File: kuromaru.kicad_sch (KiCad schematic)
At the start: 63 parts, among them J1 USB_C_Receptacle_USB2.0, J102 Serial, J5 Conn_01x02, SW1 SW_Push, SW2 SW_Push, U1 RP2040, U2 GD25Q80CEIGR, U3 XC6210B332MR-G, U4 25LCxxx, Y1 Crystal_GND24

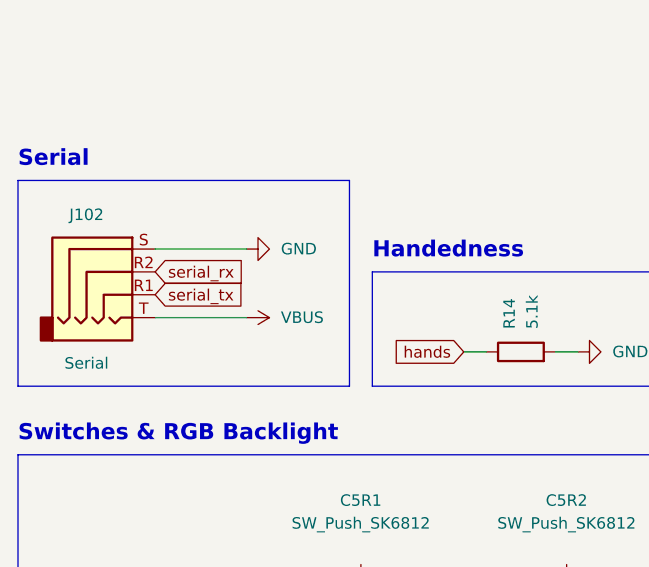
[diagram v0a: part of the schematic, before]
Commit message: Fix serial connector
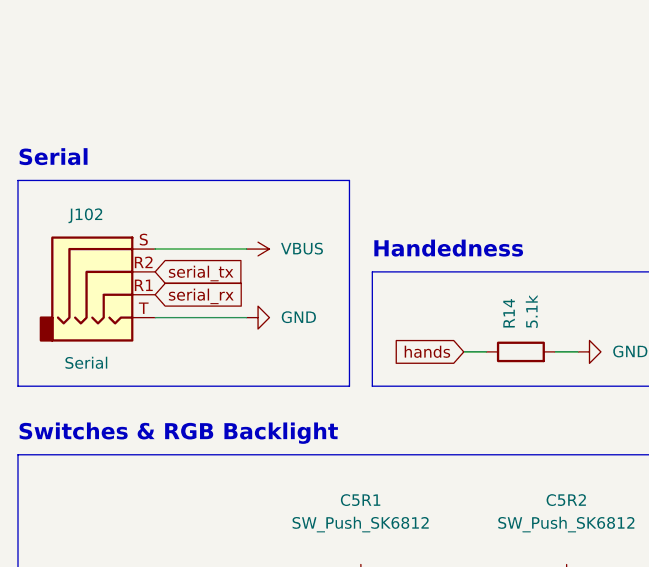
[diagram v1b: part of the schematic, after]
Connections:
- net GND: now also J102.T; no longer J102.S
- net VBUS: now also J102.S; no longer J102.T
- net serial_rx: now also J102.R1; no longer J102.R2
- net serial_tx: now also J102.R2; no longer J102.R1

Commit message: Remove RGB
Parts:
- removed C15: 1µ, Capacitor_SMD:C_0402_1005Metric, symbol Device:C
- removed R15: 300, Resistor_SMD:R_0402_1005Metric, symbol Device:R
- C1R1, C1R2, C1R3, C1R4, C2R1, C2R2, C2R4, C3R1, C3R2, C3R3, C4R1, C4R2, C4R3, C5R2, C5R3: footprint local-libraries:delay_SW_MX_RGB -> (none); symbol delay_SW_MX_RGB:SW_Push_SK6812 -> Switch:SW_Push
- C2R3, C5R1: value SW_Push_SK6812 -> (none); footprint local-libraries:delay_SW_MX_RGB -> (none); symbol delay_SW_MX_RGB:SW_Push_SK6812 -> Switch:SW_Push
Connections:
- net rgb_din is gone; now on net switch_c1r1: U1.2 (GPIO0)
- net +3V3: no longer C1R1.1 (VDD), C1R2.1 (VDD), C1R3.1 (VDD), C1R4.1 (VDD), C2R1.1 (VDD), C2R2.1 (VDD), C2R3.1 (VDD), C2R4.1 (VDD), C3R1.1 (VDD), C3R2.1 (VDD), C3R3.1 (VDD), C4R1.1 (VDD), C4R2.1 (VDD), C4R3.1 (VDD), C5R1.1 (VDD), C5R2.1 (VDD), C5R3.1 (VDD)
- net GND: now also C1R1.1, C1R2.1, C1R3.1, C1R4.1, C2R1.1, C2R2.1, C2R3.1, C2R4.1, C3R1.1, C3R2.1, C3R3.1, C4R1.1, C4R2.1, C4R3.1, C5R1.1, C5R2.1, C5R3.1; no longer C1R1.3 (GND), C1R1.5, C1R2.3 (GND), C1R2.5, C1R3.3 (GND), C1R3.5, C1R4.3 (GND), C1R4.5, C2R1.3 (GND), C2R1.5, C2R2.3 (GND), C2R2.5, C2R3.3 (GND), C2R3.5, C2R4.3 (GND), C2R4.5, C3R1.3 (GND), C3R1.5, C3R2.3 (GND), C3R2.5, C3R3.3 (GND), C3R3.5, C4R1.3 (GND), C4R1.5, C4R2.3 (GND), C4R2.5, C4R3.3 (GND), C4R3.5, C5R1.3 (GND), C5R1.5, C5R2.3 (GND), C5R2.5, C5R3.3 (GND), C5R3.5
- net switch_c1r1: now also C1R1.2; no longer C1R1.6, U1.3 (GPIO1)
- net switch_c1r2: now also C1R2.2, U1.11 (GPIO8); no longer C1R2.6, U1.12 (GPIO9)
- net switch_c1r4: now also C1R4.2; no longer C1R4.6
- net switch_c2r1: now also C2R1.2, U1.3 (GPIO1); no longer C2R1.6, U1.4 (GPIO2)
- net switch_c2r2: now also C2R2.2, U1.9 (GPIO7); no longer C2R2.6, U1.11 (GPIO8)
- net switch_c2r3: now also C2R3.2, U1.16 (GPIO13); no longer C2R3.6, U1.17 (GPIO14)
- net switch_c2r4: now also C2R4.2; no longer C2R4.6
- net switch_c3r1: now also C3R1.2, U1.4 (GPIO2); no longer C3R1.6, U1.5 (GPIO3)
- net switch_c3r2: now also C3R2.2, U1.8 (GPIO6); no longer C3R2.6, U1.9 (GPIO7)
- net switch_c3r3: now also C3R3.2, U1.15 (GPIO12); no longer C3R3.6, U1.16 (GPIO13)
- net switch_c4r1: now also C4R1.2, U1.5 (GPIO3); no longer C4R1.6, U1.6 (GPIO4)
- net switch_c4r2: now also C4R2.2, U1.7 (GPIO5); no longer C4R2.6, U1.8 (GPIO6)
- net switch_c4r3: now also C4R3.2, U1.14 (GPIO11); no longer C4R3.6, U1.15 (GPIO12)
- net switch_c5r1: now also C5R1.2, U1.6 (GPIO4); no longer C5R1.6, U1.7 (GPIO5)
- net switch_c5r2: now also C5R2.2, U1.12 (GPIO9); no longer C5R2.6, U1.13 (GPIO10)
- net switch_c5r3: now also C5R3.2, U1.13 (GPIO10); no longer C5R3.6, U1.14 (GPIO11)
- net oled_cs: now reaches C1R3.2
- net oled_cs: now also U1.17 (GPIO14); no longer C2R4.4 (DIN)
- net switch_c1r3 renamed GPIO15
- net GPIO15: no longer C1R3.6
- no-connect marks 6 -> 5
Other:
- note added: "Switches"
- note removed: "Switches & RGB Backlight"
